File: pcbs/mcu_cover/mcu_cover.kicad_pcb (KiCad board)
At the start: 2 copper layers, 20.2 x 58.7 mm, 2 parts

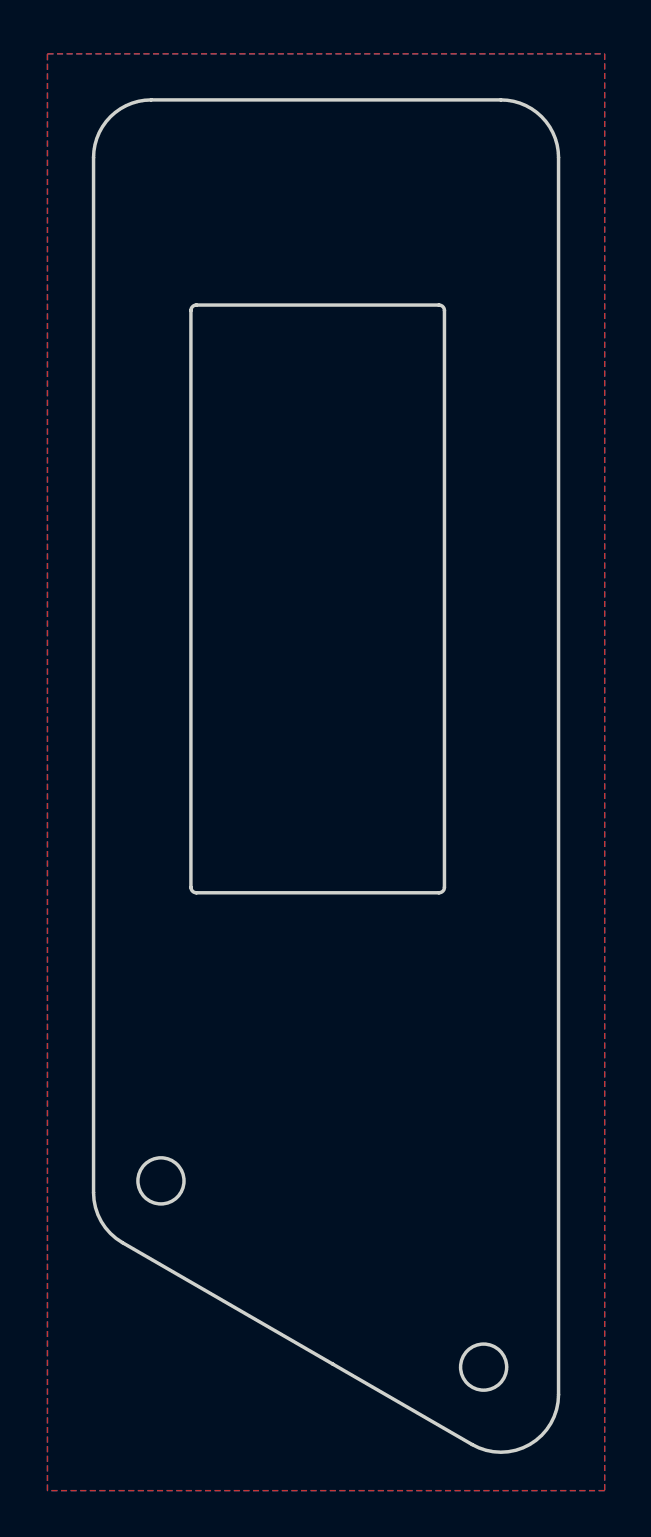
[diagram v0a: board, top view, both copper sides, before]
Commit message: update generated files
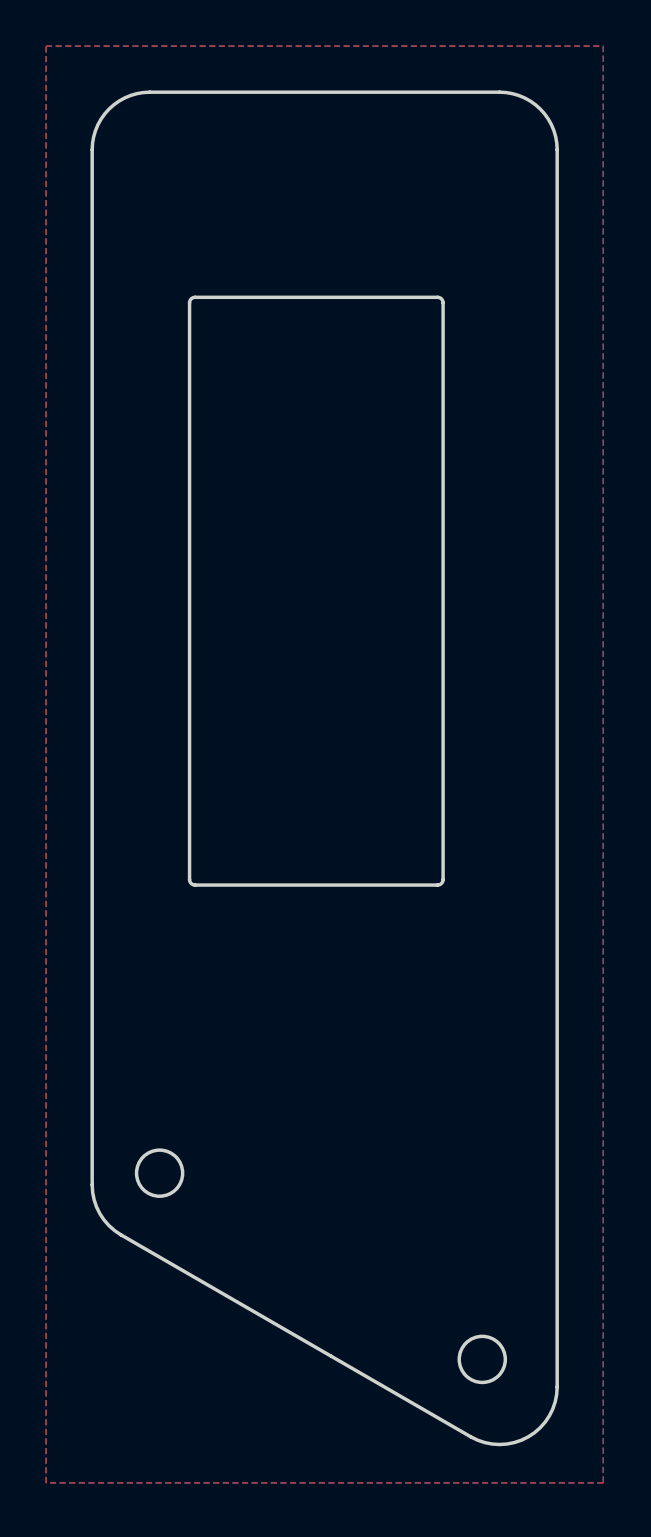
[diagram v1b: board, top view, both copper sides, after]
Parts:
- moved MH1 0.34 mm to (149.4, 86.0)
- moved MH2 0.34 mm to (163.4, 94.1)
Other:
- outline, holes or cut-outs redrawn
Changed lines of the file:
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@@
   (title_block
     (title "mcu_cover")
-    (date "2025-11-19")
+    (date "2025-11-21")
     (rev "1")
     (company "curtis bollinger")
@@
   (footprint "ceoloide:mounting_hole_npth"
     (layer "F.Cu")
-    (at 149.48162050000002 86.38459739999999 0)
+    (at 149.4225801 86.0497628 0)
     (property "Reference" "MH1"
       (at 0 2.55 0)
@@
   (footprint "ceoloide:mounting_hole_npth"
     (layer "F.Cu")
-    (at 163.48162050000002 94.46459739999999 0)
+    (at 163.4225801 94.1297628 0)
     (property "Reference" "MH2"
       (at 0 2.55 0)
@@
     )
   )
-  (gr_line (start 166.73162050000002 95.65746367967114) (end 166.73162050000002 41.9845974) (layer Edge.Cuts) (stroke (width 0.15) (type default)))
-(gr_line (start 164.23162050000002 39.4845974) (end 149.05712050000002 39.4845974) (layer Edge.Cuts) (stroke (width 0.15) (type default)))
-(gr_line (start 146.55712050000002 86.89647361252233) (end 146.55712050000002 41.9845974) (layer Edge.Cuts) (stroke (width 0.15) (type default)))
-(gr_line (start 147.8071205 89.06153711252232) (end 156.93419337992236 94.33105509502948) (layer Edge.Cuts) (stroke (width 0.15) (type default)))
-(gr_line (start 162.98162049826797 97.82252717867114) (end 156.9341984 94.33104639999999) (layer Edge.Cuts) (stroke (width 0.15) (type default)))
-(gr_arc (start 166.73162050000002 41.9845974) (mid 165.9993875 40.2168304) (end 164.23162050000002 39.4845974) (layer Edge.Cuts) (stroke (width 0.15) (type default)))
-(gr_arc (start 149.05712050000002 39.4845974) (mid 147.28935350000003 40.2168304) (end 146.55712050000002 41.9845974) (layer Edge.Cuts) (stroke (width 0.15) (type default)))
-(gr_arc (start 146.55712050000002 86.89647361252233) (mid 146.89205700000002 88.14647361252233) (end 147.80712050000002 89.06153711252233) (layer Edge.Cuts) (stroke (width 0.15) (type default)))
-(gr_arc (start 162.98162050000002 97.82252717967114) (mid 165.48162050000002 97.82252717967114) (end 166.73162050000002 95.65746367967114) (layer Edge.Cuts) (stroke (width 0.15) (type default)))
-(gr_line (start 151.02162050000004 73.88459739999999) (end 161.54162050000002 73.88459739999999) (layer Edge.Cuts) (stroke (width 0.15) (type default)))
-(gr_line (start 161.78162050000003 73.6445974) (end 161.78162050000003 48.62459739999999) (layer Edge.Cuts) (stroke (width 0.15) (type default)))
-(gr_line (start 161.54162050000002 48.38459739999999) (end 151.02162050000004 48.38459739999999) (layer Edge.Cuts) (stroke (width 0.15) (type default)))
-(gr_line (start 150.78162050000003 48.62459739999999) (end 150.78162050000003 73.6445974) (layer Edge.Cuts) (stroke (width 0.15) (type default)))
-(gr_arc (start 161.54162050000002 73.88459739999999) (mid 161.7113261 73.814303) (end 161.78162050000003 73.6445974) (layer Edge.Cuts) (stroke (width 0.15) (type default)))
-(gr_arc (start 161.78162050000003 48.62459739999999) (mid 161.7113261 48.45489179999999) (end 161.54162050000002 48.38459739999999) (layer Edge.Cuts) (stroke (width 0.15) (type default)))
-(gr_arc (start 151.02162050000004 48.38459739999999) (mid 150.85191490000005 48.45489179999999) (end 150.78162050000003 48.62459739999999) (layer Edge.Cuts) (stroke (width 0.15) (type default)))
-(gr_arc (start 150.78162050000003 73.6445974) (mid 150.85191490000005 73.814303) (end 151.02162050000004 73.88459739999999) (layer Edge.Cuts) (stroke (width 0.15) (type default)))
-(gr_circle (center 149.48162050000002 86.38459739999999) (end 150.48162050000002 86.38459739999999) (layer Edge.Cuts) (stroke (width 0.15) (type default)) (fill none))
-(gr_circle (center 163.48162050000002 94.46459739999999) (end 164.48162050000002 94.46459739999999) (layer Edge.Cuts) (stroke (width 0.15) (type default)) (fill none))
+  (gr_line (start 166.6725801 95.32262907967116) (end 166.6725801 41.649762800000005) (layer Edge.Cuts) (stroke (width 0.15) (type default)))
+(gr_line (start 164.1725801 39.149762800000005) (end 148.9980801 39.149762800000005) (layer Edge.Cuts) (stroke (width 0.15) (type default)))
+(gr_line (start 146.4980801 86.56163901252233) (end 146.4980801 41.649762800000005) (layer Edge.Cuts) (stroke (width 0.15) (type default)))
+(gr_line (start 147.74808010000004 88.72670251252235) (end 156.87515297992238 93.9962204950295) (layer Edge.Cuts) (stroke (width 0.15) (type default)))
+(gr_line (start 162.92258009826799 97.48769257867117) (end 156.875158 93.9962118) (layer Edge.Cuts) (stroke (width 0.15) (type default)))
+(gr_arc (start 166.6725801 41.649762800000005) (mid 165.9403471 39.881995800000006) (end 164.1725801 39.149762800000005) (layer Edge.Cuts) (stroke (width 0.15) (type default)))
+(gr_arc (start 148.9980801 39.149762800000005) (mid 147.23031310000002 39.881995800000006) (end 146.4980801 41.649762800000005) (layer Edge.Cuts) (stroke (width 0.15) (type default)))
+(gr_arc (start 146.4980801 86.56163901252233) (mid 146.8330166 87.81163901252233) (end 147.7480801 88.72670251252234) (layer Edge.Cuts) (stroke (width 0.15) (type default)))
+(gr_arc (start 162.9225801 97.48769257967116) (mid 165.4225801 97.48769257967116) (end 166.6725801 95.32262907967116) (layer Edge.Cuts) (stroke (width 0.15) (type default)))
+(gr_line (start 150.96258010000003 73.5497628) (end 161.4825801 73.5497628) (layer Edge.Cuts) (stroke (width 0.15) (type default)))
+(gr_line (start 161.72258010000002 73.3097628) (end 161.72258010000002 48.2897628) (layer Edge.Cuts) (stroke (width 0.15) (type default)))
+(gr_line (start 161.4825801 48.049762799999996) (end 150.96258010000003 48.049762799999996) (layer Edge.Cuts) (stroke (width 0.15) (type default)))
+(gr_line (start 150.72258010000002 48.2897628) (end 150.72258010000002 73.3097628) (layer Edge.Cuts) (stroke (width 0.15) (type default)))
+(gr_arc (start 161.4825801 73.5497628) (mid 161.6522857 73.4794684) (end 161.72258010000002 73.3097628) (layer Edge.Cuts) (stroke (width 0.15) (type default)))
+(gr_arc (start 161.72258010000002 48.2897628) (mid 161.6522857 48.1200572) (end 161.4825801 48.049762799999996) (layer Edge.Cuts) (stroke (width 0.15) (type default)))
+(gr_arc (start 150.96258010000003 48.049762799999996) (mid 150.79287450000004 48.1200572) (end 150.72258010000002 48.2897628) (layer Edge.Cuts) (stroke (width 0.15) (type default)))
+(gr_arc (start 150.72258010000002 73.3097628) (mid 150.79287450000004 73.4794684) (end 150.96258010000003 73.5497628) (layer Edge.Cuts) (stroke (width 0.15) (type default)))
+(gr_circle (center 149.4225801 86.0497628) (end 150.4225801 86.0497628) (layer Edge.Cuts) (stroke (width 0.15) (type default)) (fill none))
+(gr_circle (center 163.4225801 94.1297628) (end 164.4225801 94.1297628) (layer Edge.Cuts) (stroke (width 0.15) (type default)) (fill none))
   (zone
     (net 1)
@@
     (polygon
       (pts
-        (xy 144.55712050000002 37.4845974)
-        (xy 168.73162050000002 37.4845974)
-        (xy 168.73162050000002 99.82252717867114)
-        (xy 144.55712050000002 99.82252717867114)
+        (xy 144.4980801 37.149762800000005)
+        (xy 168.6725801 37.149762800000005)
+        (xy 168.6725801 99.48769257867117)
+        (xy 144.4980801 99.48769257867117)
       )
     )
@@
     (polygon
       (pts
-        (xy 144.55712050000002 37.4845974)
-        (xy 168.73162050000002 37.4845974)
-        (xy 168.73162050000002 99.82252717867114)
-        (xy 144.55712050000002 99.82252717867114)
+        (xy 144.4980801 37.149762800000005)
+        (xy 168.6725801 37.149762800000005)
+        (xy 168.6725801 99.48769257867117)
+        (xy 144.4980801 99.48769257867117)
       )
     )

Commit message: update generated files
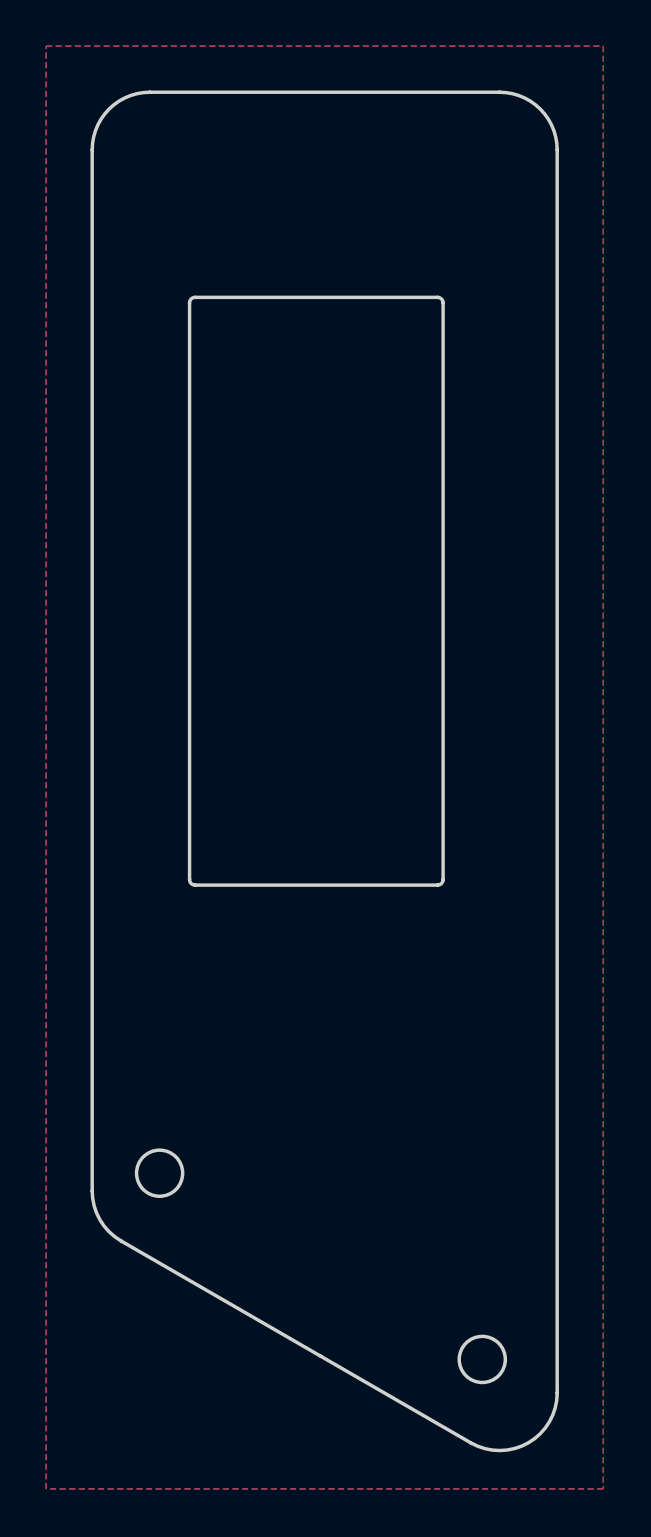
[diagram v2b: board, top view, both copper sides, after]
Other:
- board size 20.2 x 58.7 mm -> 20.2 x 58.9 mm
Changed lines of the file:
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@@
   (footprint "ceoloide:mounting_hole_npth"
     (layer "F.Cu")
-    (at 149.4225801 86.0497628 0)
+    (at 149.4228753 86.05143690000001 0)
     (property "Reference" "MH1"
       (at 0 2.55 0)
@@
   (footprint "ceoloide:mounting_hole_npth"
     (layer "F.Cu")
-    (at 163.4225801 94.1297628 0)
+    (at 163.4228753 94.13143690000001 0)
     (property "Reference" "MH2"
       (at 0 2.55 0)
@@
     )
   )
-  (gr_line (start 166.6725801 95.32262907967116) (end 166.6725801 41.649762800000005) (layer Edge.Cuts) (stroke (width 0.15) (type default)))
-(gr_line (start 164.1725801 39.149762800000005) (end 148.9980801 39.149762800000005) (layer Edge.Cuts) (stroke (width 0.15) (type default)))
-(gr_line (start 146.4980801 86.56163901252233) (end 146.4980801 41.649762800000005) (layer Edge.Cuts) (stroke (width 0.15) (type default)))
-(gr_line (start 147.74808010000004 88.72670251252235) (end 156.87515297992238 93.9962204950295) (layer Edge.Cuts) (stroke (width 0.15) (type default)))
-(gr_line (start 162.92258009826799 97.48769257867117) (end 156.875158 93.9962118) (layer Edge.Cuts) (stroke (width 0.15) (type default)))
-(gr_arc (start 166.6725801 41.649762800000005) (mid 165.9403471 39.881995800000006) (end 164.1725801 39.149762800000005) (layer Edge.Cuts) (stroke (width 0.15) (type default)))
-(gr_arc (start 148.9980801 39.149762800000005) (mid 147.23031310000002 39.881995800000006) (end 146.4980801 41.649762800000005) (layer Edge.Cuts) (stroke (width 0.15) (type default)))
-(gr_arc (start 146.4980801 86.56163901252233) (mid 146.8330166 87.81163901252233) (end 147.7480801 88.72670251252234) (layer Edge.Cuts) (stroke (width 0.15) (type default)))
-(gr_arc (start 162.9225801 97.48769257967116) (mid 165.4225801 97.48769257967116) (end 166.6725801 95.32262907967116) (layer Edge.Cuts) (stroke (width 0.15) (type default)))
-(gr_line (start 150.96258010000003 73.5497628) (end 161.4825801 73.5497628) (layer Edge.Cuts) (stroke (width 0.15) (type default)))
-(gr_line (start 161.72258010000002 73.3097628) (end 161.72258010000002 48.2897628) (layer Edge.Cuts) (stroke (width 0.15) (type default)))
-(gr_line (start 161.4825801 48.049762799999996) (end 150.96258010000003 48.049762799999996) (layer Edge.Cuts) (stroke (width 0.15) (type default)))
-(gr_line (start 150.72258010000002 48.2897628) (end 150.72258010000002 73.3097628) (layer Edge.Cuts) (stroke (width 0.15) (type default)))
-(gr_arc (start 161.4825801 73.5497628) (mid 161.6522857 73.4794684) (end 161.72258010000002 73.3097628) (layer Edge.Cuts) (stroke (width 0.15) (type default)))
-(gr_arc (start 161.72258010000002 48.2897628) (mid 161.6522857 48.1200572) (end 161.4825801 48.049762799999996) (layer Edge.Cuts) (stroke (width 0.15) (type default)))
-(gr_arc (start 150.96258010000003 48.049762799999996) (mid 150.79287450000004 48.1200572) (end 150.72258010000002 48.2897628) (layer Edge.Cuts) (stroke (width 0.15) (type default)))
-(gr_arc (start 150.72258010000002 73.3097628) (mid 150.79287450000004 73.4794684) (end 150.96258010000003 73.5497628) (layer Edge.Cuts) (stroke (width 0.15) (type default)))
-(gr_circle (center 149.4225801 86.0497628) (end 150.4225801 86.0497628) (layer Edge.Cuts) (stroke (width 0.15) (type default)) (fill none))
-(gr_circle (center 163.4225801 94.1297628) (end 164.4225801 94.1297628) (layer Edge.Cuts) (stroke (width 0.15) (type default)) (fill none))
+  (gr_line (start 166.6728753 95.58411090098006) (end 166.6728753 41.65143690000001) (layer Edge.Cuts) (stroke (width 0.15) (type default)))
+(gr_line (start 164.1728753 39.15143690000001) (end 148.9983753 39.15143690000001) (layer Edge.Cuts) (stroke (width 0.15) (type default)))
+(gr_line (start 146.4983753 86.82312083799832) (end 146.4983753 41.65143690000001) (layer Edge.Cuts) (stroke (width 0.15) (type default)))
+(gr_line (start 147.74837529999996 88.98818433799829) (end 156.42544817890752 93.99789469678733) (layer Edge.Cuts) (stroke (width 0.15) (type default)))
+(gr_line (start 162.9228752982679 97.74917439998006) (end 156.4254532 93.997886) (layer Edge.Cuts) (stroke (width 0.15) (type default)))
+(gr_arc (start 166.6728753 41.65143690000001) (mid 165.94064229999998 39.88366990000001) (end 164.1728753 39.15143690000001) (layer Edge.Cuts) (stroke (width 0.15) (type default)))
+(gr_arc (start 148.9983753 39.15143690000001) (mid 147.2306083 39.88366990000001) (end 146.4983753 41.65143690000001) (layer Edge.Cuts) (stroke (width 0.15) (type default)))
+(gr_arc (start 146.4983753 86.82312083799832) (mid 146.8333118 88.07312083799832) (end 147.7483753 88.98818433799832) (layer Edge.Cuts) (stroke (width 0.15) (type default)))
+(gr_arc (start 162.9228753 97.74917440098007) (mid 165.4228753 97.74917440098007) (end 166.6728753 95.58411090098006) (layer Edge.Cuts) (stroke (width 0.15) (type default)))
+(gr_line (start 150.9628753 73.55143690000001) (end 161.4828753 73.55143690000001) (layer Edge.Cuts) (stroke (width 0.15) (type default)))
+(gr_line (start 161.7228753 73.31143690000002) (end 161.7228753 48.291436900000015) (layer Edge.Cuts) (stroke (width 0.15) (type default)))
+(gr_line (start 161.4828753 48.05143690000001) (end 150.9628753 48.05143690000001) (layer Edge.Cuts) (stroke (width 0.15) (type default)))
+(gr_line (start 150.7228753 48.291436900000015) (end 150.7228753 73.31143690000002) (layer Edge.Cuts) (stroke (width 0.15) (type default)))
+(gr_arc (start 161.4828753 73.55143690000001) (mid 161.65258089999998 73.48114250000002) (end 161.7228753 73.31143690000002) (layer Edge.Cuts) (stroke (width 0.15) (type default)))
+(gr_arc (start 161.7228753 48.291436900000015) (mid 161.65258089999998 48.121731300000015) (end 161.4828753 48.05143690000001) (layer Edge.Cuts) (stroke (width 0.15) (type default)))
+(gr_arc (start 150.9628753 48.05143690000001) (mid 150.79316970000002 48.121731300000015) (end 150.7228753 48.291436900000015) (layer Edge.Cuts) (stroke (width 0.15) (type default)))
+(gr_arc (start 150.7228753 73.31143690000002) (mid 150.79316970000002 73.48114250000002) (end 150.9628753 73.55143690000001) (layer Edge.Cuts) (stroke (width 0.15) (type default)))
+(gr_circle (center 149.4228753 86.05143690000001) (end 150.4228753 86.05143690000001) (layer Edge.Cuts) (stroke (width 0.15) (type default)) (fill none))
+(gr_circle (center 163.4228753 94.13143690000001) (end 164.4228753 94.13143690000001) (layer Edge.Cuts) (stroke (width 0.15) (type default)) (fill none))
   (zone
     (net 1)
@@
     (polygon
       (pts
-        (xy 144.4980801 37.149762800000005)
-        (xy 168.6725801 37.149762800000005)
-        (xy 168.6725801 99.48769257867117)
-        (xy 144.4980801 99.48769257867117)
+        (xy 144.4983753 37.15143690000001)
+        (xy 168.6728753 37.15143690000001)
+        (xy 168.6728753 99.74917439998006)
+        (xy 144.4983753 99.74917439998006)
       )
     )
@@
     (polygon
       (pts
-        (xy 144.4980801 37.149762800000005)
-        (xy 168.6725801 37.149762800000005)
-        (xy 168.6725801 99.48769257867117)
-        (xy 144.4980801 99.48769257867117)
+        (xy 144.4983753 37.15143690000001)
+        (xy 168.6728753 37.15143690000001)
+        (xy 168.6728753 99.74917439998006)
+        (xy 144.4983753 99.74917439998006)
       )
     )
